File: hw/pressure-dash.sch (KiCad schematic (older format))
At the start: 29 parts, among them SW1 SW_Push

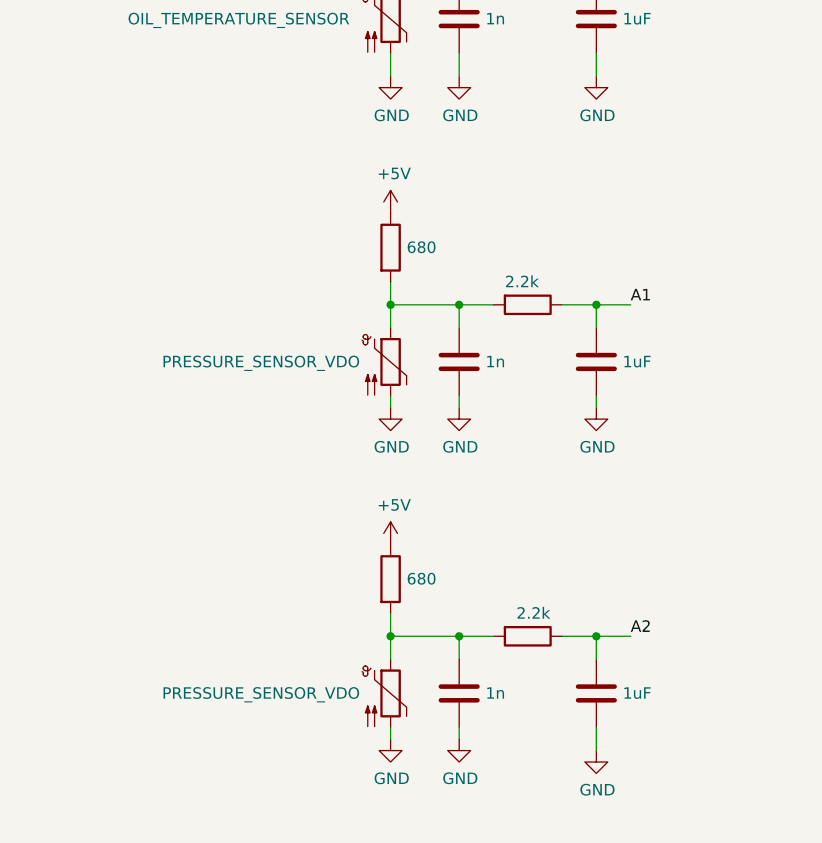
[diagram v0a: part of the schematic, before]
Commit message: Update schematic
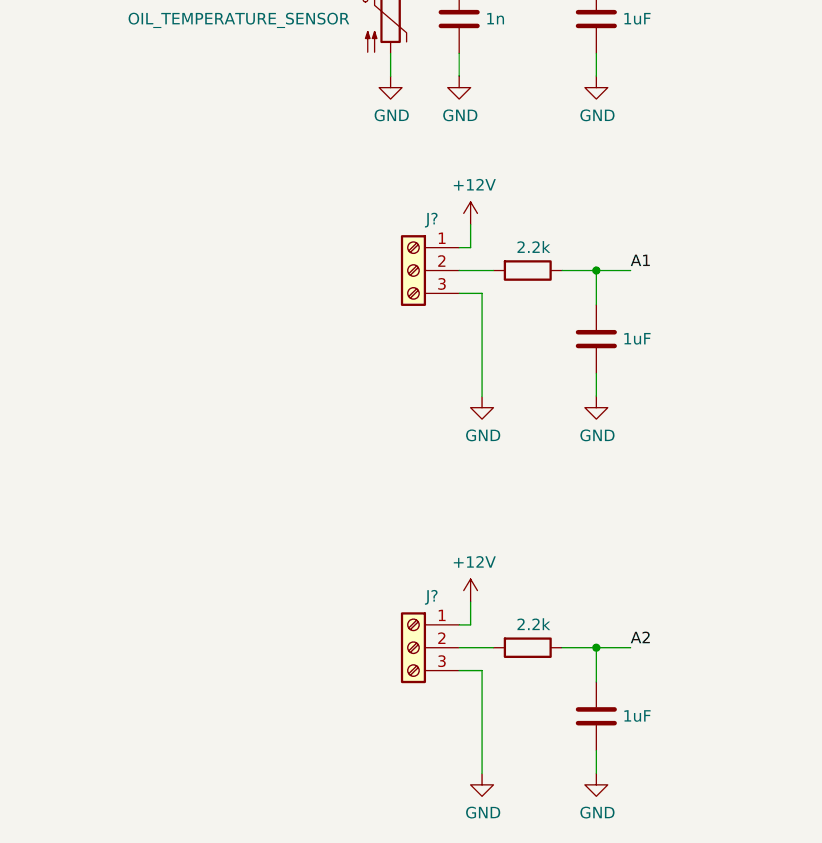
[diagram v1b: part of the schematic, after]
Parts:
- removed C? (x2): 1uF, symbol Device:C
- removed C? (x2): 1n, symbol Device:C
- removed PRESSURE_SENSOR_VDO (x2): Thermistor_PTC, symbol Device:Thermistor_PTC
- removed R? (x2): 2.2k, symbol Device:R
- removed R? (x2): 680, symbol Device:R
- added C? (x2): 1uF, symbol Device:C
- added J? (x2): Screw_Terminal_01x03, symbol Connector:Screw_Terminal_01x03
- added R? (x2): 2.2k, symbol Device:R
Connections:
- net +12V: now also J?.1 (Pin_1), J?.1 (Pin_1)
- net A1: now also C?.1, R?.1
- net A2: now also C?.1, R?.1
- net GND: now also C?.2, C?.2, J?.3 (Pin_3), J?.3 (Pin_3)
- new net: J?.2 (Pin_2), R?.2 (x2)
